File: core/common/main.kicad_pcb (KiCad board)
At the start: 2 copper layers, 99.1 x 49.8 mm, 11 parts, among them P1 CONN_01X05, P2 CONN_01X03, P3 CONN_01X02, P4 CONN_01X02, P5 CONN_01X28, P7 CONN_01X28, P8 CONN_01X28, U1 NDSL_DPad, U2 NDSL_SS, U3 N900_Keyboard, U4 N900_Keyboard

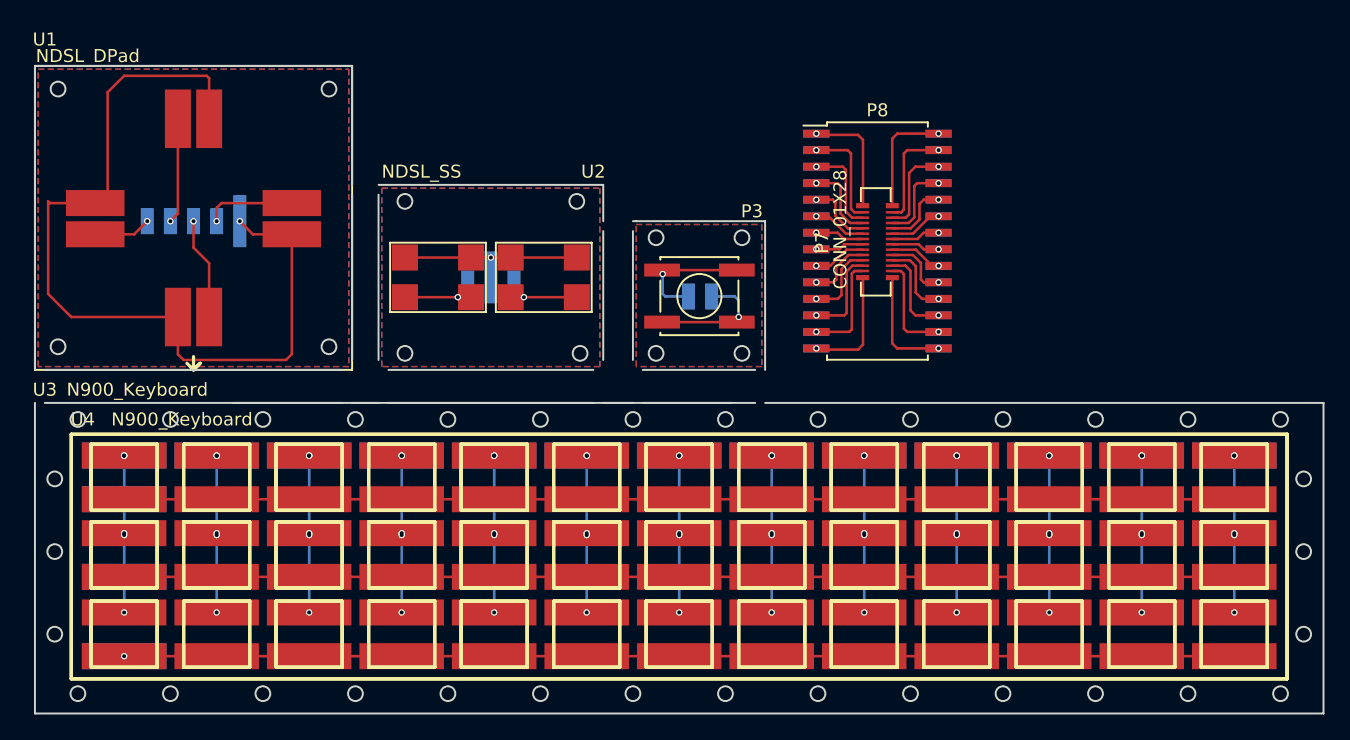
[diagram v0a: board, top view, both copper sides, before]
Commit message: updated n900 pcb
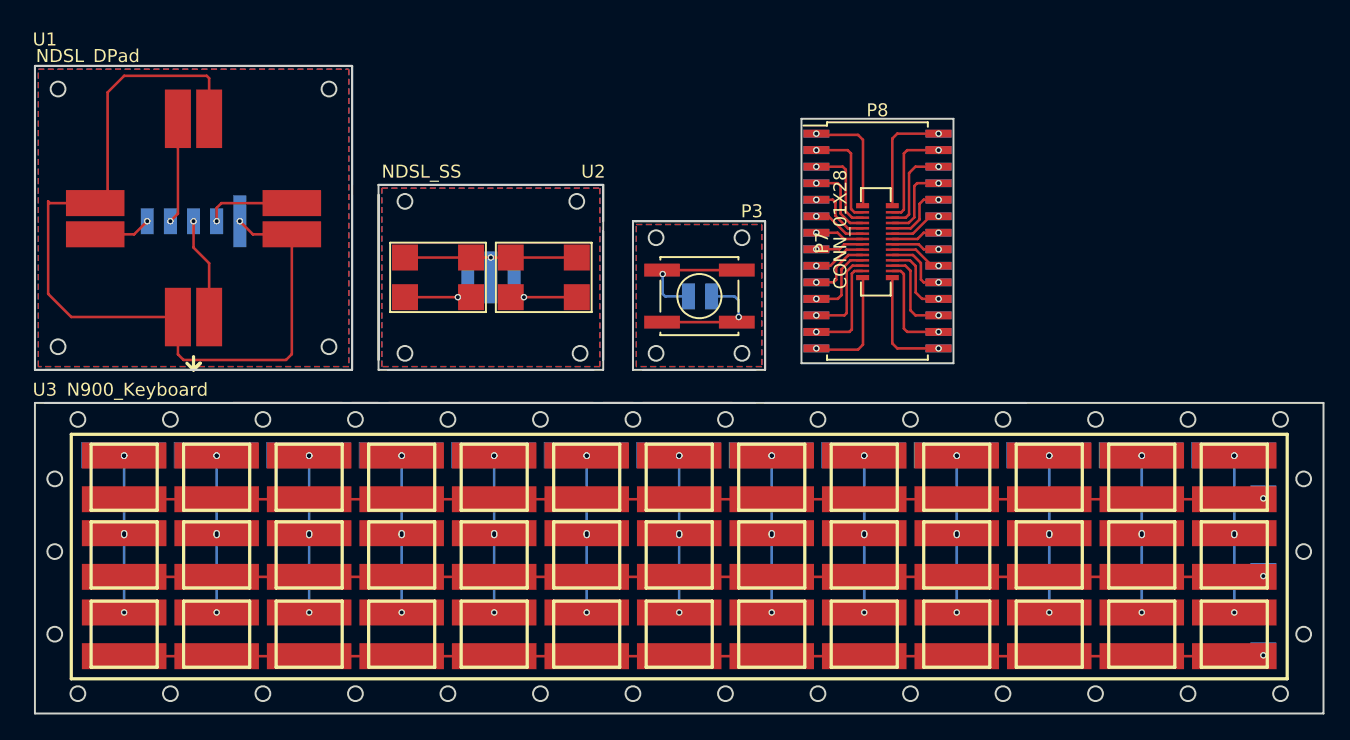
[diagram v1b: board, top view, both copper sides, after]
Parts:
- U4: moved to B.Cu
- moved U4 6.55 mm to (109.2, 145.5), turned to 180 degrees
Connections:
- U4 pad 1: K1 -> K13
- U4 pad 10: K10 -> K4
- U4 pad 11: K11 -> K3
- U4 pad 12: K12 -> K2
- U4 pad 13: K13 -> K1
- U4 pad 2: K2 -> K12
- U4 pad 3: K3 -> K11
- U4 pad 4: K4 -> K10
- U4 pad 5: K5 -> K9
- U4 pad 6: K6 -> K8
- U4 pad 8: K8 -> K6
- U4 pad 9: K9 -> K5
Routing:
- net K16: track 85.3 -> 87.6 mm
- net K14: track 85.3 -> 87.6 mm, vias 0 -> 1
- net K15: track 85.3 -> 87.6 mm, vias 0 -> 1
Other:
- outline, holes or cut-outs redrawn
